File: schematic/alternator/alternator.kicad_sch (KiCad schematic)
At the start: 10 parts, among them J1 NMEA2k, J2 Shunt, J3 Alt Temp, J4 Batt/Field, Q1 NMOS, Q2 PMOS, U1 ESP32-DEVKITC-32E, U2 TJA1051T, U3 INA260, U4 XL1509-5.0

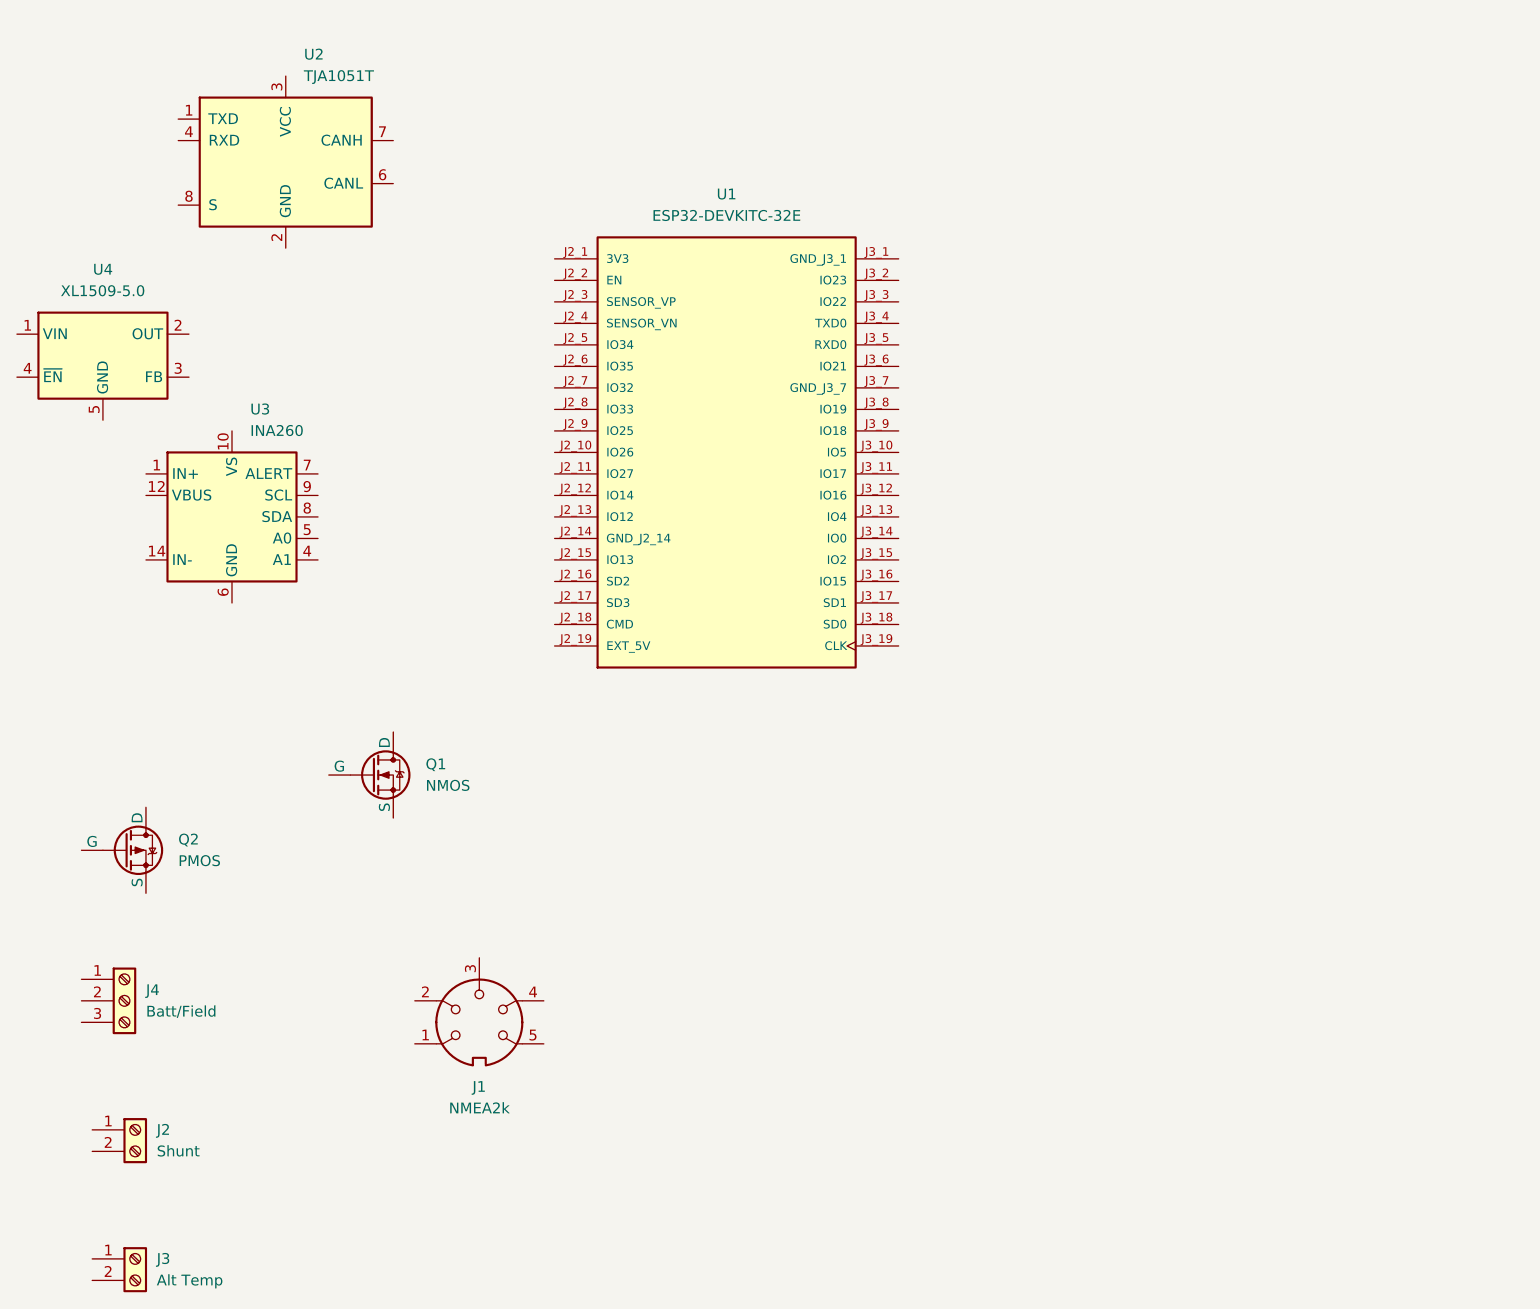
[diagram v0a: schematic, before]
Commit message: xx
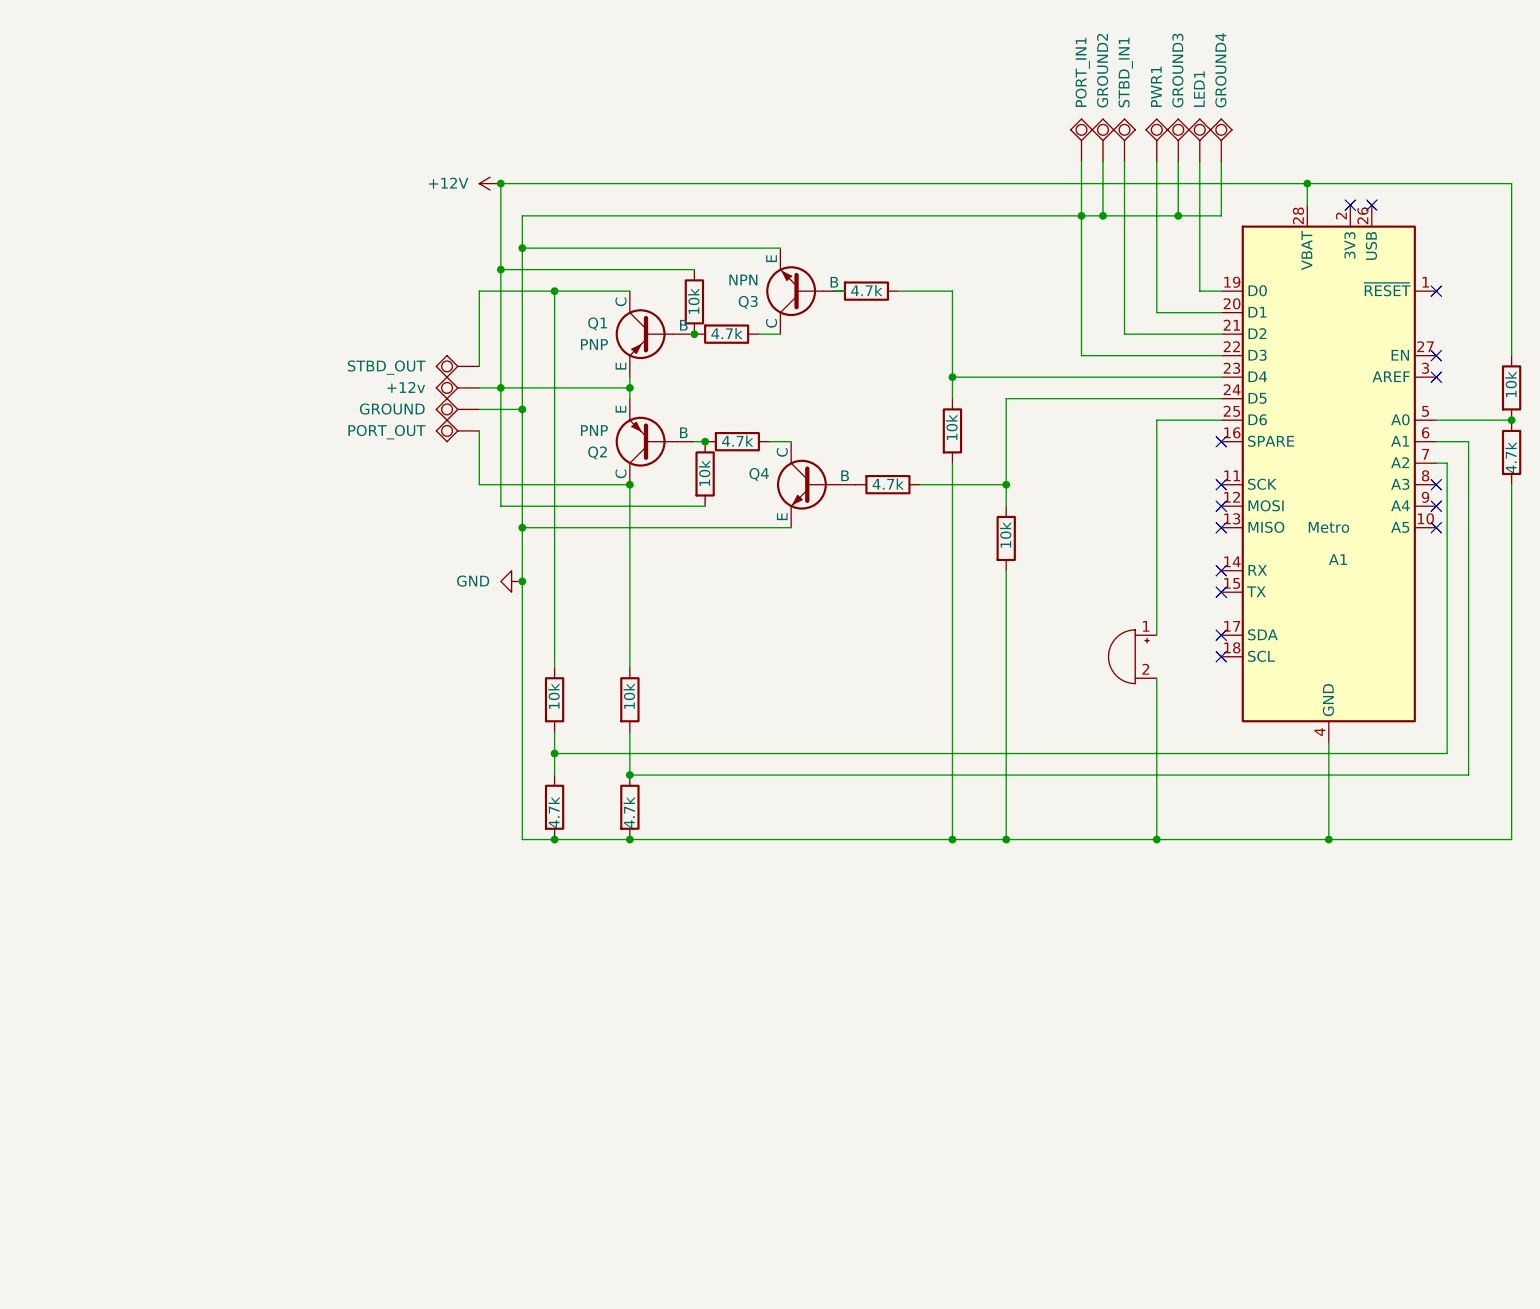
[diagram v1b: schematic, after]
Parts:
- removed J1: NMEA2k, symbol Connector:DIN-5
- removed J2: Shunt, symbol Connector:Screw_Terminal_01x02
- removed J3: Alt Temp, symbol Connector:Screw_Terminal_01x02
- removed J4: Batt/Field, symbol Connector:Screw_Terminal_01x03
- removed Q1: NMOS, symbol Simulation_SPICE:NMOS
- removed Q2: PMOS, symbol Simulation_SPICE:PMOS
- removed U1: ESP32-DEVKITC-32E, ESP32-DEVKITC-32E:MODULE_ESP32-DEVKITC-32E, symbol ESP32-DEVKITC-32E:ESP32-DEVKITC-32E
- removed U2: TJA1051T, Package_SO:SOIC-8_3.9x4.9mm_P1.27mm, symbol Interface_CAN_LIN:TJA1051T
- removed U3: INA260, Package_SO:TSSOP-16_4.4x5mm_P0.65mm, symbol Sensor:INA260
- removed U4: XL1509-5.0, Package_SO:SOIC-8_3.9x4.9mm_P1.27mm, symbol Regulator_Switching:XL1509-5.0
- added +12v, GROUND, GROUND2, GROUND3, GROUND4, LED1, PORT_IN1, PORT_OUT, PWR1, STBD_IN1, STBD_OUT: TESTPAD, TestPoint:TestPoint_Pad_D1.5mm, symbol OLIMEX_OTHER:TESTPAD
- added A1: Metro, Module:Adafruit_Feather, symbol MCU_Module:Adafruit_Feather_Generic
- added BZ1: Buzzer, Buzzer_Beeper:Buzzer_12x9.5RM7.6, symbol Device:Buzzer
- added Q1, Q2: PNP, Package_TO_SOT_THT:TO-92L_Inline, symbol Simulation_SPICE:PNP
- added Q3, Q4: NPN, symbol Simulation_SPICE:NPN
- added R1, R13, R14, R3, R5, R8, R9: 10k, Resistor_THT:R_Axial_DIN0207_L6.3mm_D2.5mm_P7.62mm_Horizontal, symbol Device:R
- added R10, R11, R12, R15, R2, R4, R7: 4.7k, Resistor_THT:R_Axial_DIN0207_L6.3mm_D2.5mm_P7.62mm_Horizontal, symbol Device:R
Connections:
- new net: Q3.1 (C), R15.1
- new net: Q3.2 (B), R7.2
- new net: PORT_OUT.1 (Pad), Q2.1 (C), R3.1
- new net: A1.6 (A1), R3.2, R4.1
- new net: Q1.1 (C), R1.1, STBD_OUT.1 (Pad)
- new net: Q1.2 (B), R15.2, R5.2
- new net: A1.24 (D5), R11.1, R14.1
- new net: Q4.2 (B), R11.2
- new net: A1.19 (D0), LED1.1 (Pad)
- new net: A1.21 (D2), STBD_IN1.1 (Pad)
- new net: Q4.1 (C), R12.1
- new net: A1.20 (D1), PWR1.1 (Pad)
- new net: A1.23 (D4), R13.1, R7.1
- new net: Q2.2 (B), R12.2, R8.1
- new net: A1.7 (A2), R1.2, R2.1
- new net: A1.25 (D6), BZ1.1 (+)
- new net: A1.5 (A0), R10.1, R9.2
- new net +12V: +12v.1 (Pad), A1.28 (VBAT), Q1.3 (E), Q2.3 (E), R5.1, R8.2, R9.1
- new net GND: A1.22 (D3), A1.4 (GND), BZ1.2 (-), GROUND.1 (Pad), GROUND2.1 (Pad), GROUND3.1 (Pad), GROUND4.1 (Pad), PORT_IN1.1 (Pad), Q3.3 (E), Q4.3 (E), R10.2, R13.2, R14.2, R2.2, R4.2
- no-connect marks 0 -> 16
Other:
- company: (none) -> David Ros
- title: (none) -> Bow Thruster Controller
